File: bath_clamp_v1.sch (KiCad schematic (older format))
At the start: 20 parts, among them U10 LP2951-3.3_SOIC, U6 24AA025UID, U7 LM337L_SO8, U9 MCP1804x-3302xOT

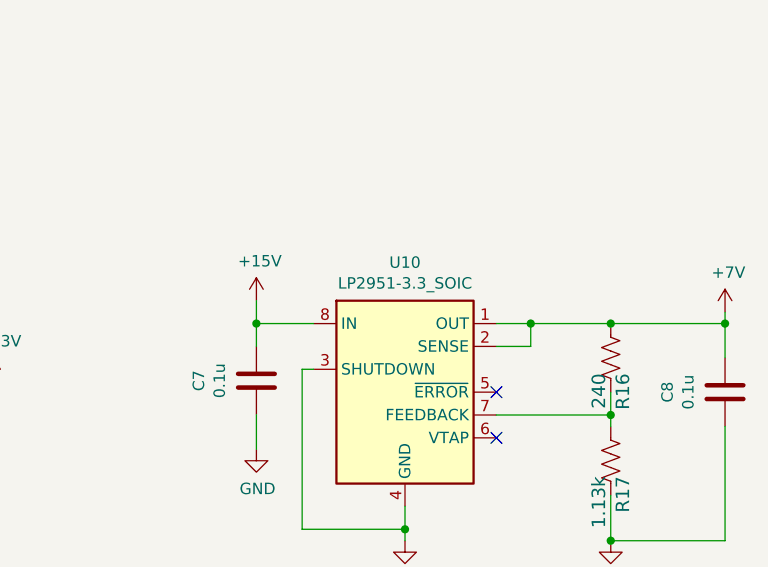
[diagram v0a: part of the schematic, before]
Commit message: readme updates
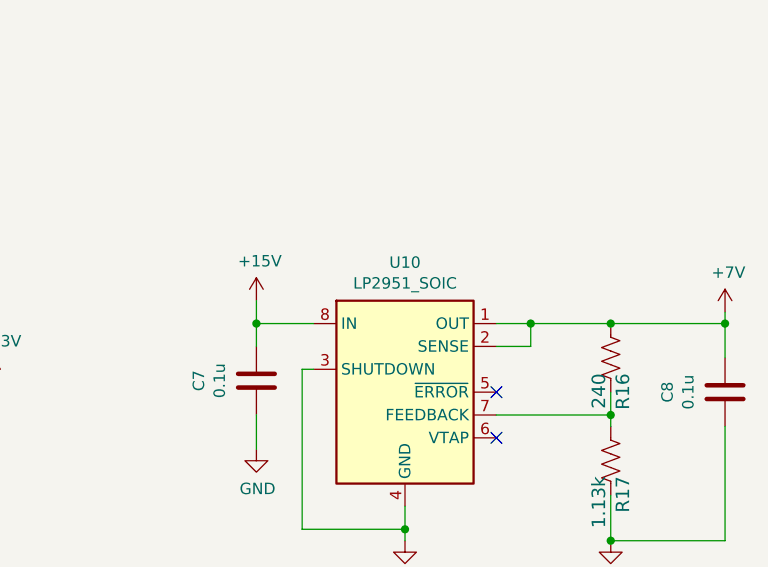
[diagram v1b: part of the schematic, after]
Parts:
- C4: Manf# CC0603MRX7R8BB104 -> CL10B104KA8NNWC; Tolerance 20% -> 10%
- U10: value LP2951-3.3_SOIC -> LP2951_SOIC; Manf# LP2951CDR2G -> LP2951ACDR2G
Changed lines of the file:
@@
 F 2 "Capacitor_SMD:C_0603_1608Metric" H 4938 2900 50  0001 C CNN
 F 3 "~" H 4900 3050 50  0001 C CNN
-F 4 "CC0603MRX7R8BB104" H 4648 3150 50  0001 C CNN "Manf#"
-F 5 "20%" H 4648 3150 50  0001 C CNN "Tolerance"
+F 4 "CL10B104KA8NNWC" H 4648 3150 50  0001 C CNN "Manf#"
+F 5 "10%" H 4648 3150 50  0001 C CNN "Tolerance"
 F 6 "25V" H 4648 3150 50  0001 C CNN "voltage"
 	1    4900 3050
@@
 P 8200 2750
 F 0 "U10" H 8200 3317 50  0000 C CNN
-F 1 "LP2951-3.3_SOIC" H 8200 3226 50  0000 C CNN
+F 1 "LP2951_SOIC" H 8200 3226 50  0000 C CNN
 F 2 "Package_SO:SOIC-8_3.9x4.9mm_P1.27mm" H 8200 2100 50  0001 C CNN
 F 3 "http://www.ti.com/lit/ds/symlink/lp2951-n.pdf" H 8200 2750 50  0001 C CNN
-F 4 "LP2951CDR2G" H 8200 3417 50  0001 C CNN "Manf#"
+F 4 "LP2951ACDR2G" H 8200 3417 50  0001 C CNN "Manf#"
 	1    8200 2750
 	1    0    0    -1
